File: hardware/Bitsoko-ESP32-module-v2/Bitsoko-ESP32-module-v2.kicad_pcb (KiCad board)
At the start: 2 copper layers, 40.6 x 27.9 mm, 3 parts, among them J1 CONN_02X10, J2 CONN_02X10, U1 ESP32-WROOM32-MODULE

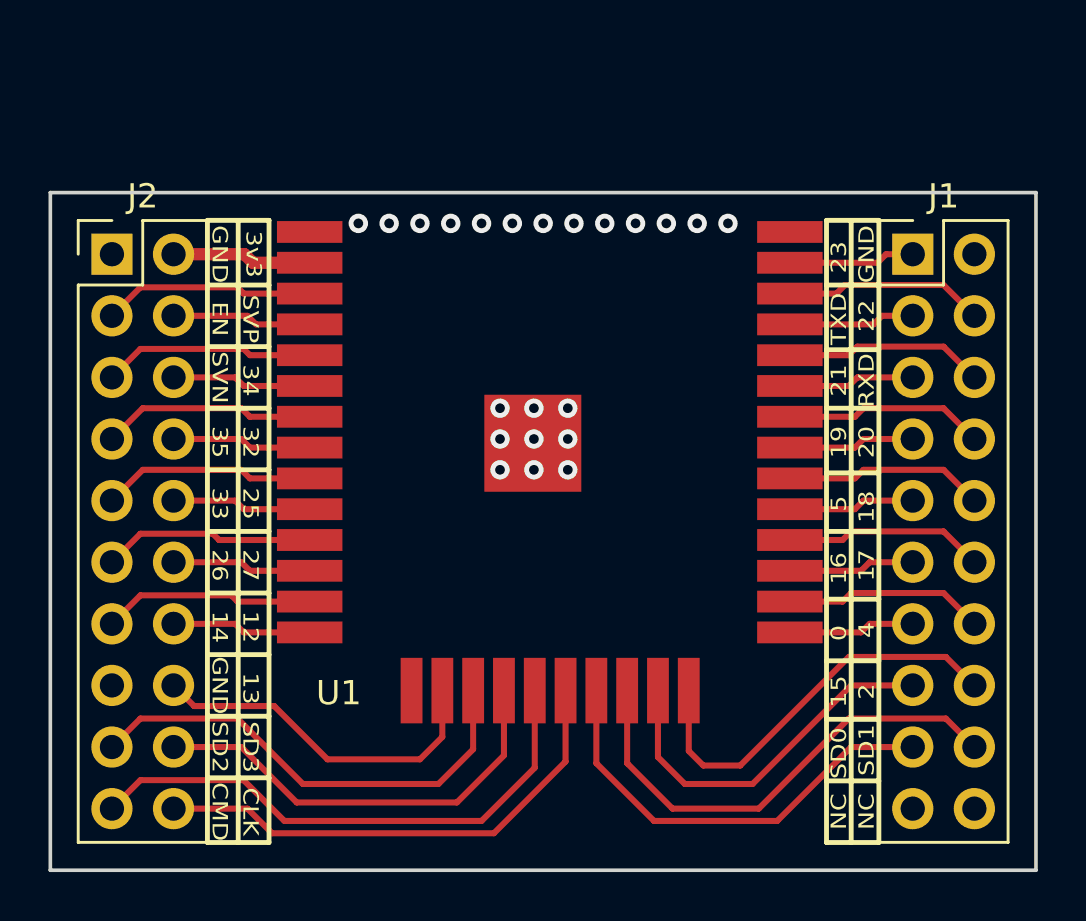
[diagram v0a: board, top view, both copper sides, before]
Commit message: Replaced pin headers with offset staggered headers from a friction fit without soldering
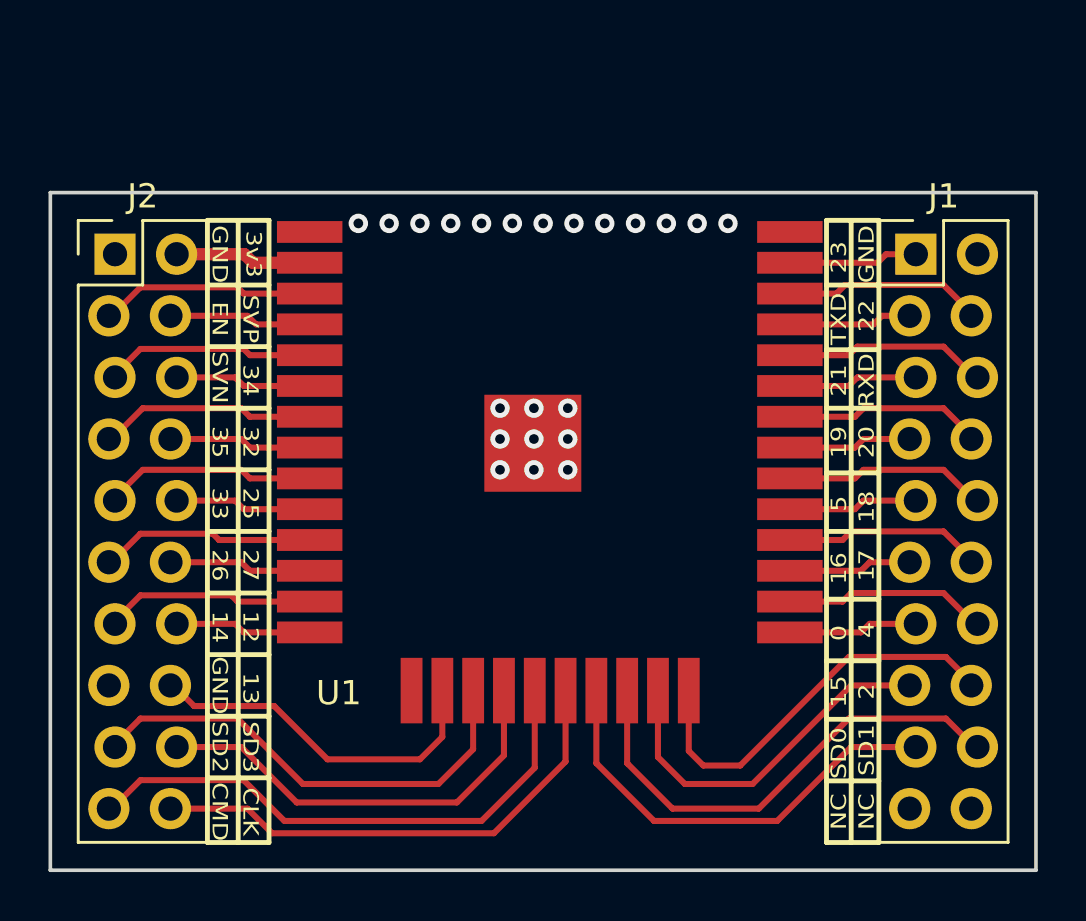
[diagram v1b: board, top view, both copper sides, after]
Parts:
- J1, J2: footprint Pin_Headers:Pin_Header_Straight_2x10_Pitch2.54mm -> narra:Pin_Header_Straight_2x10_Pitch2.54mm_staggered
